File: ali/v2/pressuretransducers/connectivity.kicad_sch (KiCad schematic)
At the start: 27 parts, among them J8 Conn_01x03, J9 Vertical Ethernet, U3 TJA1462ATK, U4 LAN8742AI, Y3 25 MHz

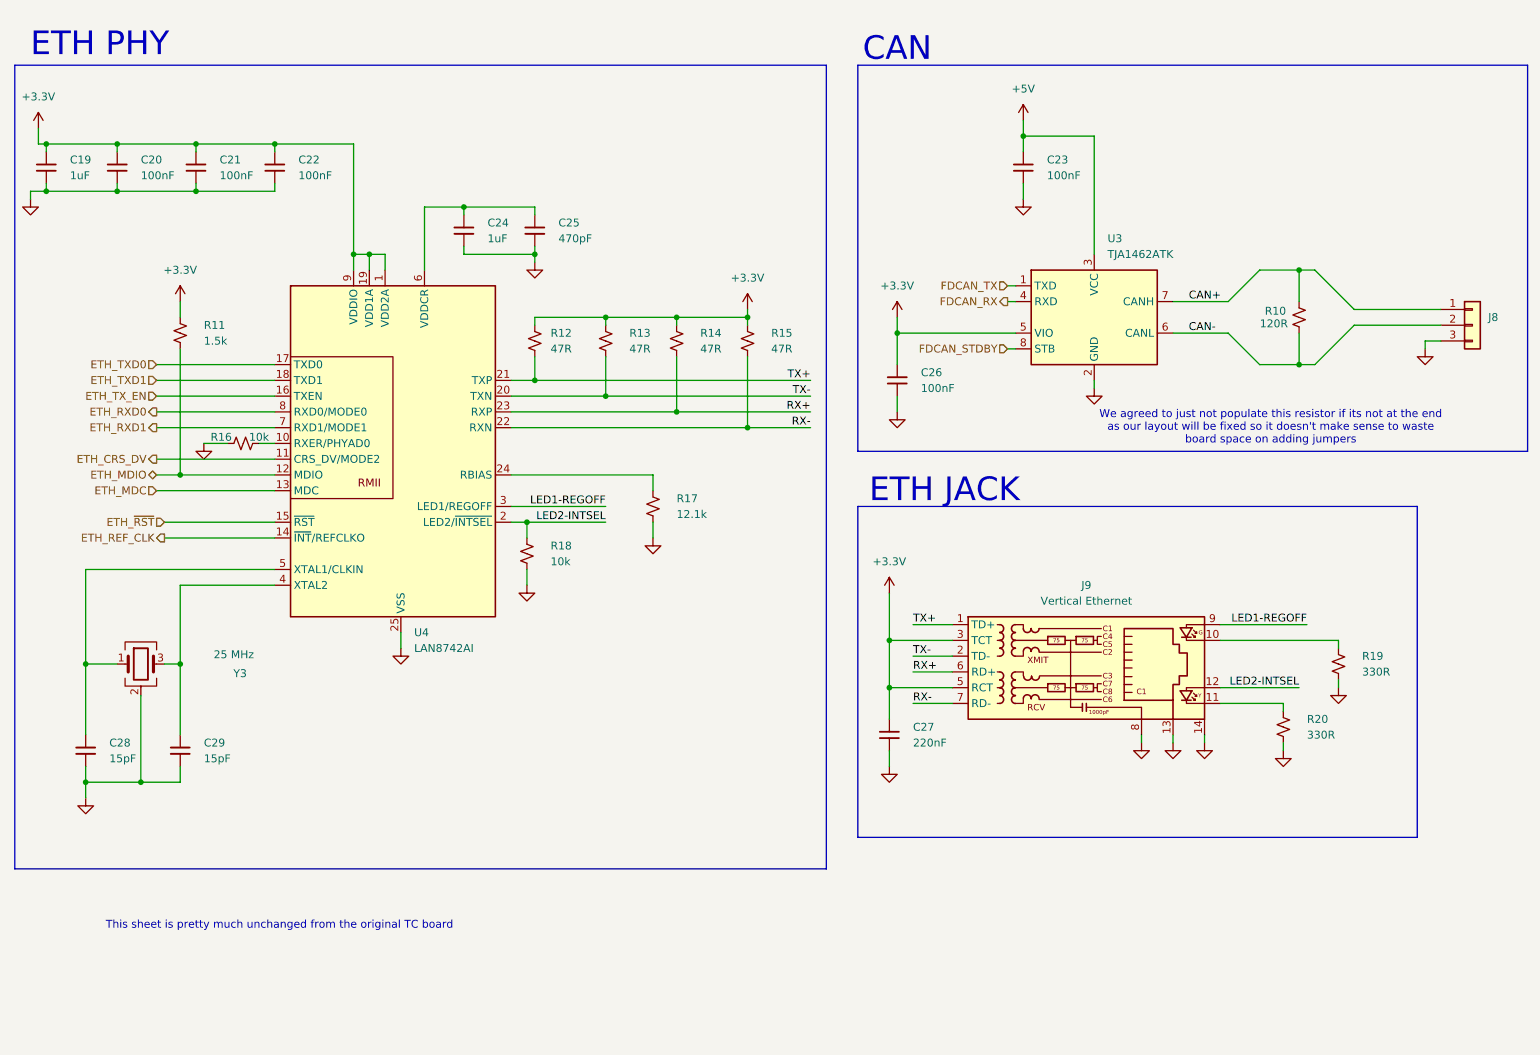
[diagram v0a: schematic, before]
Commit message: Begin prep for second board review
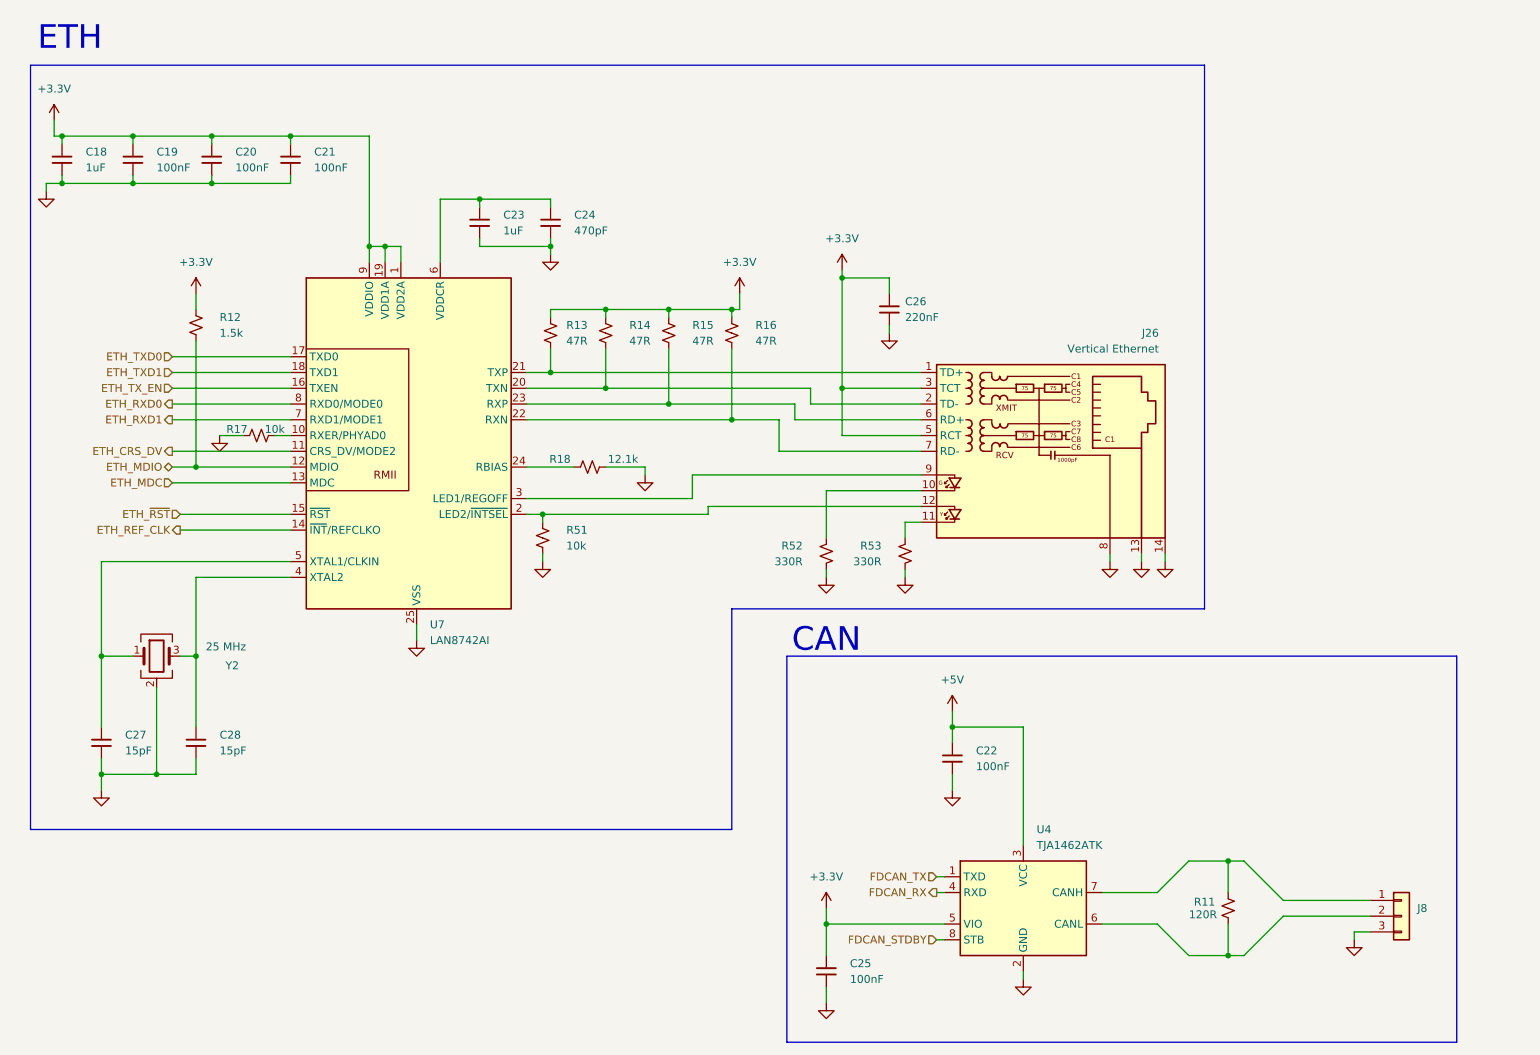
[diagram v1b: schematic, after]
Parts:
- removed C29: 15pF, APRL_Passive:C_0603, symbol Device:C_Small
- removed J9: Vertical Ethernet, APRL_Connector:RJ45_Hanrun_HY951180A_Vertical, symbol APRL_Connector:RJ45_Hanrun_HY951180A
- removed R10: 120R, APRL_Passive:R_0603, symbol Device:R_Small_US
- removed R19, R20: 330R, APRL_Passive:R_0603, symbol Device:R_Small_US
- removed U3: TJA1462ATK, APRL_Package_QFN:HVSON-8-1EP_3x3mm_P0.65mm_EP1.6x2.4mm_ThermalVias, symbol APRL_Comms:TJA1462ATK
- removed U4: LAN8742AI, APRL_Package_QFN:VQFN-24-1EP_4x4mm_P0.5mm_EP2.5x2.5mm_ThermalVias, symbol APRL_Comms:LAN8742A
- removed Y3: 25 MHz, APRL_Passive:3225-4P-L, symbol Device:Crystal_GND24
- added C18: 1uF, APRL_Passive:C_0603, symbol Device:C_Small
- added J26: Vertical Ethernet, APRL_Connector:RJ45_Hanrun_HY951180A_Vertical, symbol APRL_Connector:RJ45_Hanrun_HY951180A
- added R51: 10k, APRL_Passive:R_0603, symbol Device:R_Small_US
- added R52, R53: 330R, APRL_Passive:R_0603, symbol Device:R_Small_US
- added U4: TJA1462ATK, APRL_Package_QFN:HVSON-8-1EP_3x3mm_P0.65mm_EP1.6x2.4mm_ThermalVias, symbol APRL_Comms:TJA1462ATK
- added U7: LAN8742AI, APRL_Package_QFN:VQFN-24-1EP_4x4mm_P0.5mm_EP2.5x2.5mm_ThermalVias, symbol APRL_Comms:LAN8742A
- added Y2: 25 MHz, APRL_Passive:3225-4P-L, symbol Device:Crystal_GND24
- C19: value 1uF -> 100nF; MPN GRM188D72A105KE01 -> GRM188R72A104KA35
- C23: value 100nF -> 1uF; MPN GRM188R72A104KA35 -> GRM188D72A105KE01
- C24: value 1uF -> 470pF; MPN GRM188D72A105KE01 -> GRM1885C1H471JA01
- C25: value 470pF -> 100nF; MPN GRM1885C1H471JA01 -> GRM188R72A104KA35
- C26: value 100nF -> 220nF; MPN GRM188R72A104KA35 -> GRM188R71H224KAC4
- C27: value 220nF -> 15pF; MPN GRM188R71H224KAC4 -> GRM1885C2E150FW07
- R11: value 1.5k -> 120R; MPN RC0603FR-071K5L -> AC0603FR-07120RL
- R12: value 47R -> 1.5k; MPN RC0603FR-0747RL -> RC0603FR-071K5L
- R16: value 10k -> 47R; MPN RC0603FR-0710KL -> RC0603FR-0747RL
- R17: value 12.1k -> 10k; MPN RT0603BRD0712K1L -> RC0603FR-0710KL
- R18: value 10k -> 12.1k; MPN RC0603FR-0710KL -> RT0603BRD0712K1L
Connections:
- net TX+ is gone; now on net ETH_MDIO: R12.2
- net +3.3V: now also C25.1, R16.1, C18.1, J26.3 (TCT), J26.5 (RCT), U4.5 (VIO), U7.1 (VDD2A), U7.19 (VDD1A), U7.9 (VDDIO); no longer C22.1, C27.1, R11.1
- net +5V: now also C22.1, U4.3 (VCC); no longer C23.1
- net ETH_CRS_DV: now also U7.11 (CRS_DV/MODE2)
- net ETH_MDC: now also U7.13 (MDC)
- net ETH_MDIO: now also U7.12 (MDIO); no longer R11.2
- net ETH_REF_CLK: now also U7.14 (~{INT}/REFCLKO)
- net ETH_RXD0: now also U7.8 (RXD0/MODE0)
- net ETH_RXD1: now also U7.7 (RXD1/MODE1)
- net ETH_TXD0: now also U7.17 (TXD0)
- net ETH_TXD1: now also U7.18 (TXD1)
- net ETH_TX_EN: now also U7.16 (TXEN)
- net ETH_~{RST}: now also U7.15 (~{RST})
- net FDCAN_RX: now also U4.4 (RXD)
- net FDCAN_STDBY: now also U4.8 (STB)
- net FDCAN_TX: now also U4.1 (TXD)
- net GND: now also R17.1, C18.2, J26.13, J26.14, J26.8, R51.2, R52.2, R53.2, U4.2 (GND), U4.9 (GND), U7.25 (VSS), Y2.2 (G), Y2.4 (G); no longer R16.1, R17.2
- net at C28.1: now also U7.4 (XTAL2), Y2.3
- net at C24.1: now also C23.1, U7.6 (VDDCR); no longer C25.1
- net at R16.2: now also J26.7 (RD-), U7.22 (RXN)
- net CAN+: no longer names the net of J8.1 (Pin_1)
- net CAN+: now also R11.2, U4.7 (CANH)
- net CAN-: no longer names the net of J8.2 (Pin_2)
- net CAN-: now also R11.1, U4.6 (CANL)
- net LED2-INTSEL: no longer names the net of R18.1
- net LED2-INTSEL: now also U7.24 (RBIAS)
- net RX+: no longer names the net of R14.2
- net RX+: now also J26.2 (TD-), U7.20 (TXN)
- net RX-: no longer names the net of R15.2
- net RX-: now also J26.6 (RD+), U7.23 (RXP)
- net TX-: no longer names the net of R13.2
- net TX-: now also J26.1 (TD+), U7.21 (TXP)
- new net: J26.11, R53.1
- new net: C27.1, U7.5 (XTAL1/CLKIN), Y2.1
- new net: J26.12, R51.1, U7.2 (LED2/~{INTSEL})
- new net: J26.10, R52.1
- new net: J26.9, U7.3 (LED1/REGOFF)
- new net: R17.2, U7.10 (RXER/PHYAD0)
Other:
- note added: "ETH"
- note removed: "ETH JACK"
- note removed: "ETH PHY"
- note removed: "This sheet is pretty much unchanged from the original TC board"
- note removed: "We agreed to just not populate this resistor if its not at the end as our layout will be fixed so it doesn't make sense to waste board space on adding jumpers"
